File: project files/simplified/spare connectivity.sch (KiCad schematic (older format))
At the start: 4 parts, among them J6 Target STDC-14, U3 STM32F103CBUx

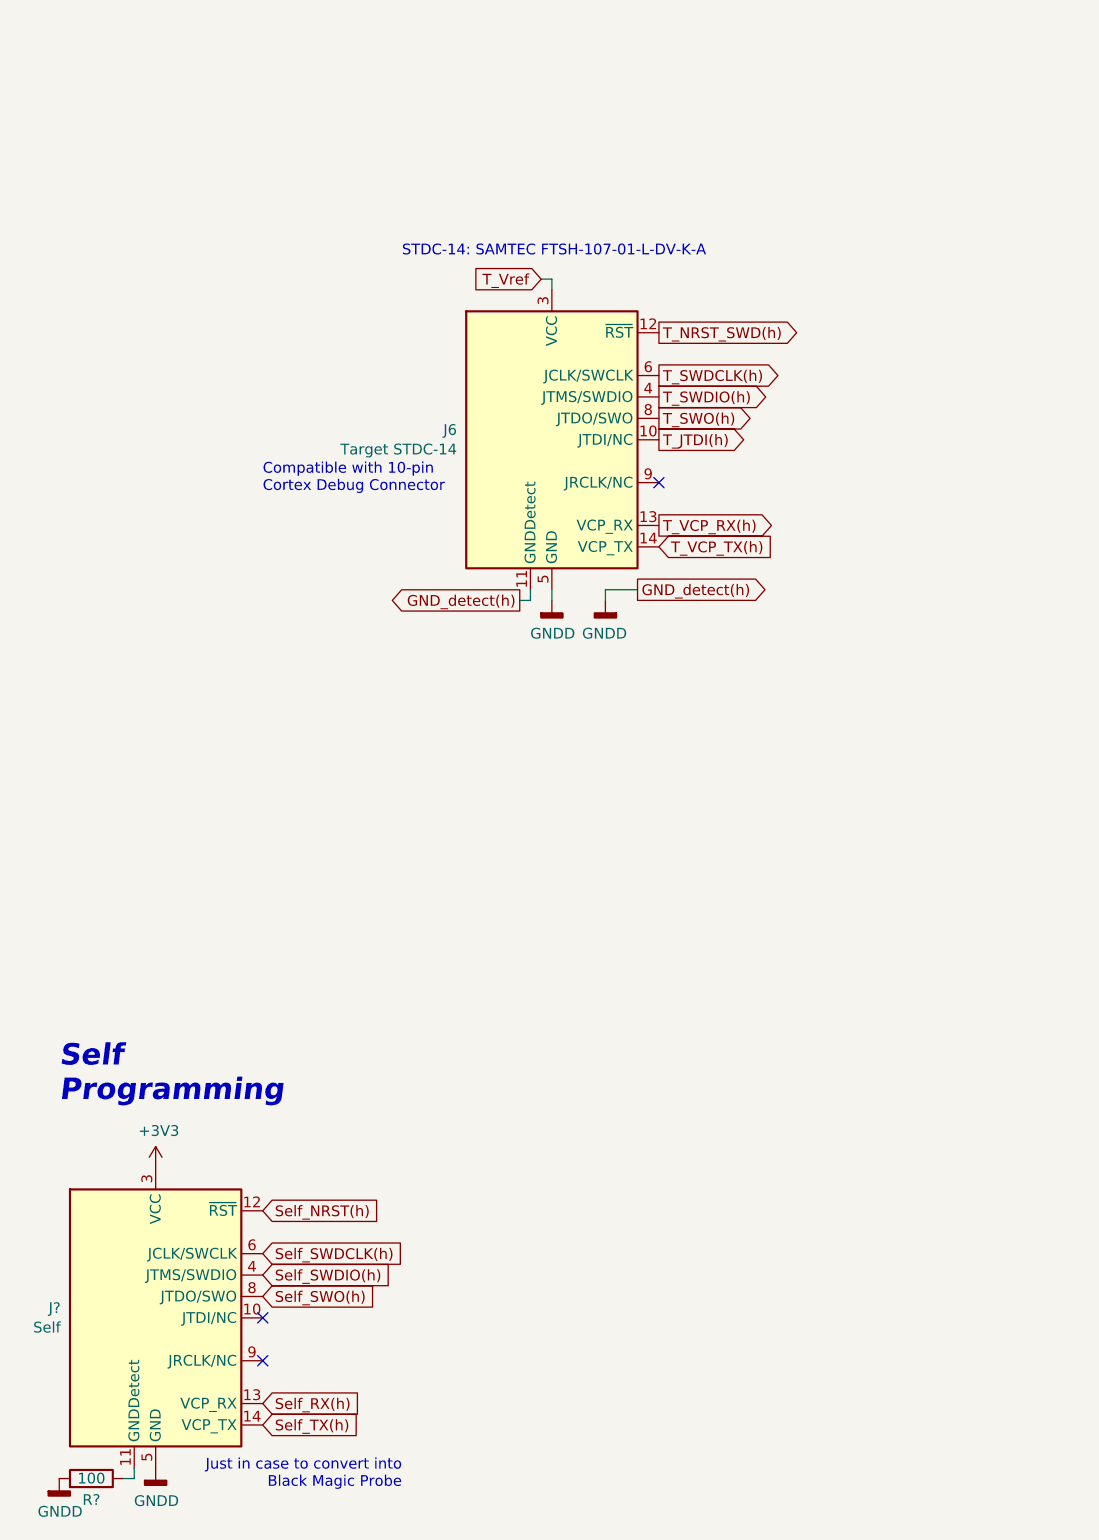
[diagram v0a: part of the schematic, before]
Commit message: re-arrangements
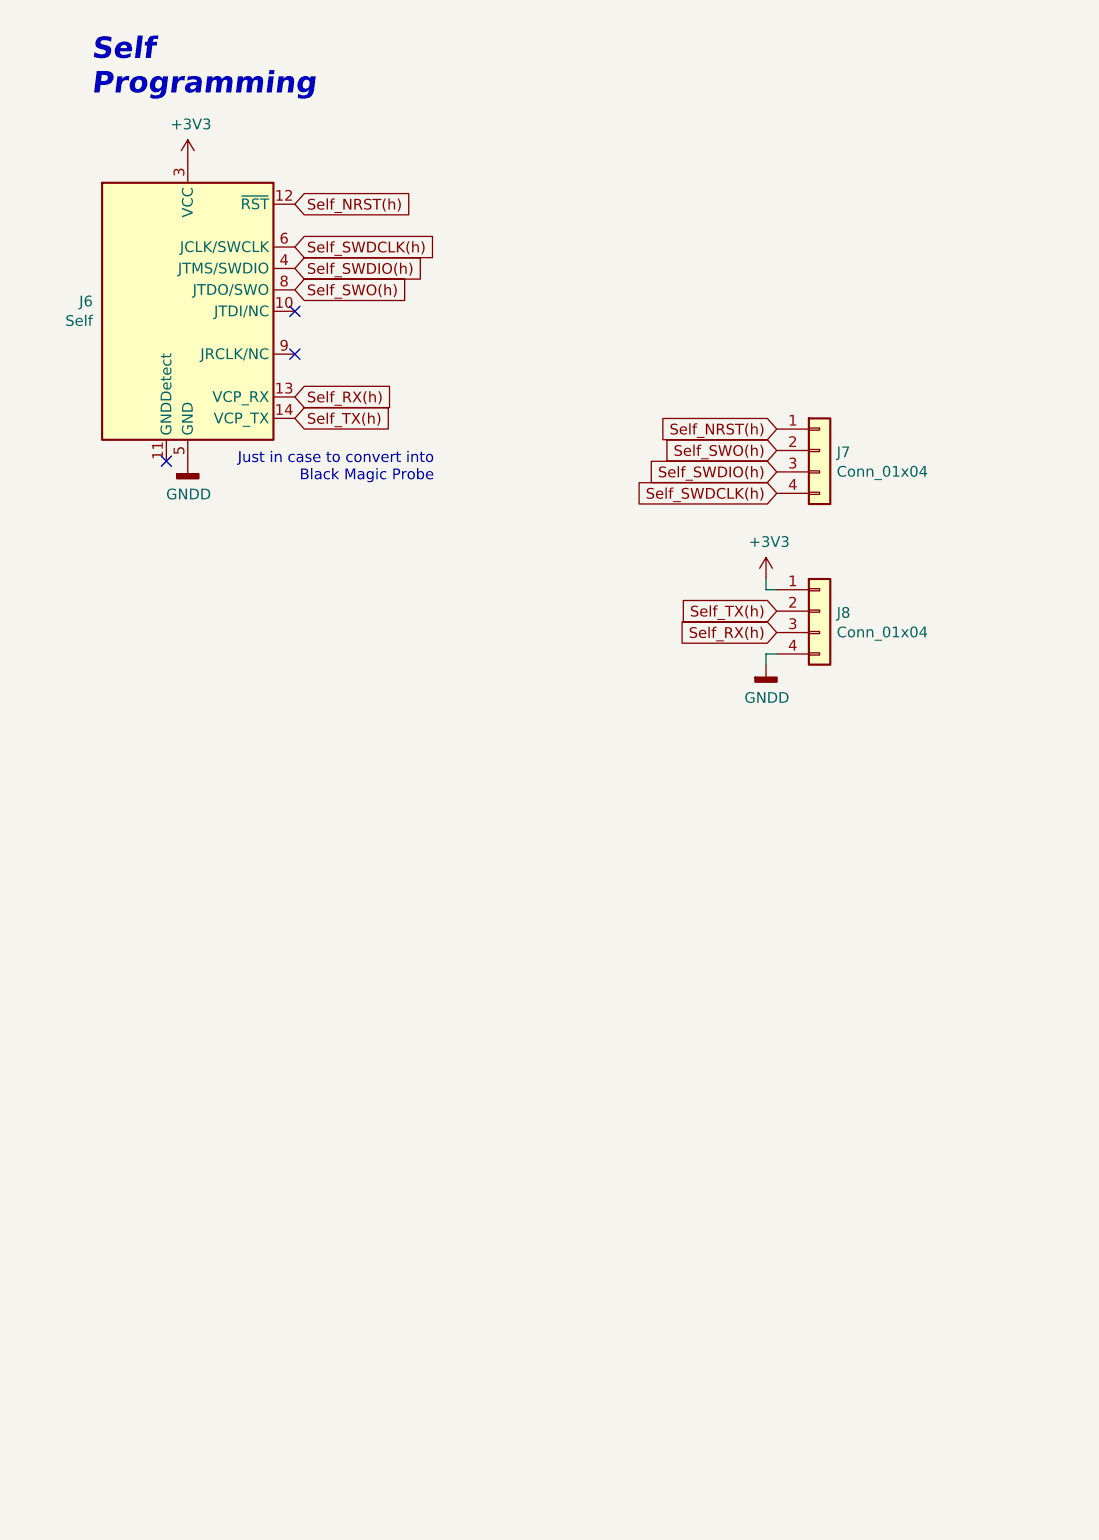
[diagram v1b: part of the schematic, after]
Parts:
- removed J6: Target STDC-14, Connector_PinHeader_1.27mm:PinHeader_2x07_P1.27mm_Vertical_SMD, symbol Connector:Conn_ST_STDC14
- removed R?: 100, Resistor_SMD:R_0603_1608Metric, symbol Device:R
- added J7, J8: Conn_01x04, Connector_PinHeader_2.54mm:PinHeader_1x04_P2.54mm_Vertical, symbol Connector_Generic:Conn_01x04
- gave numbers to parts that had none: 1
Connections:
- net +3V3: now also J8.1 (Pin_1)
- net GNDD: now also J8.4 (Pin_4)
- net Self_NRST(h): now also J7.1 (Pin_1)
- net Self_RX(h): now also J8.3 (Pin_3)
- net Self_SWDCLK(h): now also J7.4 (Pin_4)
- net Self_SWDIO(h): now also J7.3 (Pin_3)
- net Self_SWO(h): now also J7.2 (Pin_2)
- net Self_TX(h): now also J8.2 (Pin_2)
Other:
- note removed: "Compatible with 10-pin\nCortex Debug Connector"
- note removed: "STDC-14: SAMTEC FTSH-107-01-L-DV-K-A"
- moved on the sheet: J6
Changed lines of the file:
@@
 Comment4 ""
 $EndDescr
-Text GLabel 3450 2550 2    50   Output ~ 0
-T_SWO(h)
-Text GLabel 3450 2350 2    50   Output ~ 0
-T_SWDCLK(h)
-Text GLabel 3450 2150 2    50   Output ~ 0
-T_NRST_SWD(h)
-Text GLabel 3450 3150 2    50   Input ~ 0
-T_VCP_TX(h)
-Text GLabel 3450 3050 2    50   Output ~ 0
-T_VCP_RX(h)
-Text Notes 1600 2900 0    50   ~ 0
-Compatible with 10-pin\nCortex Debug Connector
-Text GLabel 3450 2450 2    50   Output ~ 0
-T_SWDIO(h)
-$Comp
-L power:GNDD #PWR?
-U 1 1 5EC35CB1
-P 2950 3400
-AR Path="/5EC35CB1" Ref="#PWR?"  Part="1"
-AR Path="/5EC31CA9/5EC35CB1" Ref="#PWR050"  Part="1"
-F 0 "#PWR050" H 2950 3150 50  0001 C CNN
-F 1 "GNDD" H 2954 3245 50  0000 C CNN
-F 2 "" H 2950 3400 50  0001 C CNN
-F 3 "" H 2950 3400 50  0001 C CNN
-	1    2950 3400
-	1    0    0    -1
-$EndComp
-Text Notes 2250 1800 0    50   ~ 0
-STDC-14: SAMTEC FTSH-107-01-L-DV-K-A
-$Comp
-L power:GNDD #PWR?
-U 1 1 5EC35CBA
-P 3200 3400
-AR Path="/5EC35CBA" Ref="#PWR?"  Part="1"
-AR Path="/5EC31CA9/5EC35CBA" Ref="#PWR051"  Part="1"
-F 0 "#PWR051" H 3200 3150 50  0001 C CNN
-F 1 "GNDD" H 3204 3245 50  0000 C CNN
-F 2 "" H 3200 3400 50  0001 C CNN
-F 3 "" H 3200 3400 50  0001 C CNN
-	1    3200 3400
-	-1   0    0    -1
-$EndComp
-Wire Wire Line
-	3350 3350 3200 3350
-Wire Wire Line
-	3200 3350 3200 3400
-Wire Wire Line
-	2800 3400 2850 3400
-Wire Wire Line
-	2850 3400 2850 3350
-Wire Wire Line
-	2950 3400 2950 3350
-NoConn ~ 3450 2850
-Text GLabel 3450 2650 2    50   Output ~ 0
-T_JTDI(h)
-$Comp
-L Connector:Conn_ST_STDC14 J?
-U 1 1 5EC35CC7
-P 2950 2650
-AR Path="/5EC35CC7" Ref="J?"  Part="1"
-AR Path="/5EC31CA9/5EC35CC7" Ref="J6"  Part="1"
-F 0 "J6" H 2507 2696 50  0000 R CNN
-F 1 "Target STDC-14" H 2507 2605 50  0000 R CNN
-F 2 "Connector_PinHeader_1.27mm:PinHeader_2x07_P1.27mm_Vertical_SMD" H 2950 2650 50  0001 C CNN
-F 3 "https://www.st.com/content/ccc/resource/technical/document/user_manual/group1/99/49/91/b6/b2/3a/46/e5/DM00526767/files/DM00526767.pdf/jcr:content/translations/en.DM00526767.pdf" V 2600 1400 50  0001 C CNN
-	1    2950 2650
-	1    0    0    -1
-$EndComp
-Wire Wire Line
-	2900 1900 2950 1900
-Wire Wire Line
-	2950 1900 2950 1950
-Text GLabel 2900 1900 0    50   Input ~ 0
-T_Vref
 Wire Wire Line
 	10050 4000 10050 3950
@@
 	9650 4000 9750 4000
 $Comp
-L power:GNDD #PWR053
+L power:GNDD #PWR055
 U 1 1 5EC6BDFB
 P 10050 4050
-F 0 "#PWR053" H 10050 3800 50  0001 C CNN
+F 0 "#PWR055" H 10050 3800 50  0001 C CNN
 F 1 "GNDD" H 10054 3895 50  0000 C CNN
 F 2 "" H 10050 4050 50  0001 C CNN
@@
 	9950 900  10050 900
 $Comp
-L power:+3.3V #PWR052
+L power:+3.3V #PWR050
 U 1 1 5EC6FD9F
 P 9850 900
-F 0 "#PWR052" H 9850 750 50  0001 C CNN
+F 0 "#PWR050" H 9850 750 50  0001 C CNN
 F 1 "+3.3V" H 9865 1073 50  0000 C CNN
 F 2 "" H 9850 900 50  0001 C CNN
@@
 	1    0    0    -1
 $EndComp
-Text GLabel 3350 3350 2    50   Output ~ 0
-GND_detect(h)
-Text GLabel 2800 3400 0    50   Output ~ 0
-GND_detect(h)
-Text Notes 2250 7550 2    50   ~ 0
+Text Notes 2400 2850 2    50   ~ 0
 Just in case to convert into\nBlack Magic Probe
-Text GLabel 1600 7250 2    50   Input ~ 0
+Text GLabel 1750 2550 2    50   Input ~ 0
 Self_TX(h)
-Text GLabel 1600 7150 2    50   Input ~ 0
+Text GLabel 1750 2450 2    50   Input ~ 0
 Self_RX(h)
 $Comp
-L power:GNDD #PWR?
+L power:GNDD #PWR052
 U 1 1 5F1BD152
-P 1100 7450
-F 0 "#PWR?" H 1100 7200 50  0001 C CNN
-F 1 "GNDD" H 1104 7295 50  0000 C CNN
-F 2 "" H 1100 7450 50  0001 C CNN
-F 3 "" H 1100 7450 50  0001 C CNN
-	1    1100 7450
-	1    0    0    -1
-$EndComp
-Text GLabel 1600 6250 2    50   Input ~ 0
+P 1250 2750
+F 0 "#PWR052" H 1250 2500 50  0001 C CNN
+F 1 "GNDD" H 1254 2595 50  0000 C CNN
+F 2 "" H 1250 2750 50  0001 C CNN
+F 3 "" H 1250 2750 50  0001 C CNN
+	1    1250 2750
+	1    0    0    -1
+$EndComp
+Text GLabel 1750 1550 2    50   Input ~ 0
 Self_NRST(h)
-NoConn ~ 1600 6950
-Text GLabel 1600 6650 2    50   Input ~ 0
+NoConn ~ 1750 2250
+Text GLabel 1750 1950 2    50   Input ~ 0
 Self_SWO(h)
-Text GLabel 1600 6450 2    50   Input ~ 0
+Text GLabel 1750 1750 2    50   Input ~ 0
 Self_SWDCLK(h)
-Text GLabel 1600 6550 2    50   Input ~ 0
+Text GLabel 1750 1850 2    50   Input ~ 0
 Self_SWDIO(h)
 $Comp
-L power:+3V3 #PWR?
+L power:+3V3 #PWR051
 U 1 1 5F1BD15D
-P 1100 6050
-F 0 "#PWR?" H 1100 5900 50  0001 C CNN
-F 1 "+3V3" H 1115 6223 50  0000 C CNN
-F 2 "" H 1100 6050 50  0001 C CNN
-F 3 "" H 1100 6050 50  0001 C CNN
-	1    1100 6050
-	1    0    0    -1
-$EndComp
-NoConn ~ 1600 6750
-$Comp
-L Connector:Conn_ST_STDC14 J?
+P 1250 1350
+F 0 "#PWR051" H 1250 1200 50  0001 C CNN
+F 1 "+3V3" H 1265 1523 50  0000 C CNN
+F 2 "" H 1250 1350 50  0001 C CNN
+F 3 "" H 1250 1350 50  0001 C CNN
+	1    1250 1350
+	1    0    0    -1
+$EndComp
+NoConn ~ 1750 2050
+$Comp
+L Connector:Conn_ST_STDC14 J6
 U 1 1 5F1BD164
-P 1100 6750
-F 0 "J?" H 657 6796 50  0000 R CNN
-F 1 "Self" H 657 6705 50  0000 R CNN
-F 2 "Connector_PinHeader_1.27mm:PinHeader_2x07_P1.27mm_Vertical_SMD" H 1100 6750 50  0001 C CNN
-F 3 "https://www.st.com/content/ccc/resource/technical/document/user_manual/group1/99/49/91/b6/b2/3a/46/e5/DM00526767/files/DM00526767.pdf/jcr:content/translations/en.DM00526767.pdf" V 750 5500 50  0001 C CNN
-	1    1100 6750
-	1    0    0    -1
-$EndComp
-Text Notes 650  5750 0    100  Italic 20
+P 1250 2050
+F 0 "J6" H 807 2096 50  0000 R CNN
+F 1 "Self" H 807 2005 50  0000 R CNN
+F 2 "Connector_PinHeader_1.27mm:PinHeader_2x07_P1.27mm_Vertical_SMD" H 1250 2050 50  0001 C CNN
+F 3 "https://www.st.com/content/ccc/resource/technical/document/user_manual/group1/99/49/91/b6/b2/3a/46/e5/DM00526767/files/DM00526767.pdf/jcr:content/translations/en.DM00526767.pdf" V 900 800 50  0001 C CNN
+	1    1250 2050
+	1    0    0    -1
+$EndComp
+Text Notes 800  1050 0    100  Italic 20
 Self\nProgramming
-$Comp
-L Device:R R?
-U 1 1 5F1BD16B
-P 800 7500
-F 0 "R?" V 700 7500 50  0000 C CNN
-F 1 "100" V 800 7500 50  0000 C CNN
-F 2 "Resistor_SMD:R_0603_1608Metric" V 730 7500 50  0001 C CNN
-F 3 "~" H 800 7500 50  0001 C CNN
-	1    800  7500
-	0    1    -1   0
-$EndComp
-$Comp
-L power:GNDD #PWR?
-U 1 1 5F1BD171
-P 650 7500
-F 0 "#PWR?" H 650 7250 50  0001 C CNN
-F 1 "GNDD" H 654 7345 50  0000 C CNN
-F 2 "" H 650 7500 50  0001 C CNN
-F 3 "" H 650 7500 50  0001 C CNN
-	1    650  7500
-	1    0    0    -1
-$EndComp
-Wire Wire Line
-	950  7500 1000 7500
-Wire Wire Line
-	1000 7500 1000 7450
+NoConn ~ 1150 2750
+$Comp
+L Connector_Generic:Conn_01x04 J7
+U 1 1 5FCDFBAC
+P 4200 2700
+F 0 "J7" H 4280 2692 50  0000 L CNN
+F 1 "Conn_01x04" H 4280 2601 50  0000 L CNN
+F 2 "Connector_PinHeader_2.54mm:PinHeader_1x04_P2.54mm_Vertical" H 4200 2700 50  0001 C CNN
+F 3 "~" H 4200 2700 50  0001 C CNN
+	1    4200 2700
+	1    0    0    -1
+$EndComp
+$Comp
+L Connector_Generic:Conn_01x04 J8
+U 1 1 5FCE032D
+P 4200 3450
+F 0 "J8" H 4280 3442 50  0000 L CNN
+F 1 "Conn_01x04" H 4280 3351 50  0000 L CNN
+F 2 "Connector_PinHeader_2.54mm:PinHeader_1x04_P2.54mm_Vertical" H 4200 3450 50  0001 C CNN
+F 3 "~" H 4200 3450 50  0001 C CNN
+	1    4200 3450
+	1    0    0    -1
+$EndComp
+Text GLabel 4000 3450 0    50   Input ~ 0
+Self_TX(h)
+Text GLabel 4000 3550 0    50   Input ~ 0
+Self_RX(h)
+$Comp
+L power:GNDD #PWR054
+U 1 1 5FCE1122
+P 3950 3700
+F 0 "#PWR054" H 3950 3450 50  0001 C CNN
+F 1 "GNDD" H 3954 3545 50  0000 C CNN
+F 2 "" H 3950 3700 50  0001 C CNN
+F 3 "" H 3950 3700 50  0001 C CNN
+	1    3950 3700
+	1    0    0    -1
+$EndComp
+$Comp
+L power:+3V3 #PWR053
+U 1 1 5FCE1839
+P 3950 3300
+F 0 "#PWR053" H 3950 3150 50  0001 C CNN
+F 1 "+3V3" H 3965 3473 50  0000 C CNN
+F 2 "" H 3950 3300 50  0001 C CNN
+F 3 "" H 3950 3300 50  0001 C CNN
+	1    3950 3300
+	1    0    0    -1
+$EndComp
+Wire Wire Line
+	4000 3350 3950 3350
+Wire Wire Line
+	3950 3350 3950 3300
+Wire Wire Line
+	4000 3650 3950 3650
+Wire Wire Line
+	3950 3650 3950 3700
+Text GLabel 4000 2700 0    50   Input ~ 0
+Self_SWO(h)
+Text GLabel 4000 2900 0    50   Input ~ 0
+Self_SWDCLK(h)
+Text GLabel 4000 2800 0    50   Input ~ 0
+Self_SWDIO(h)
+Text GLabel 4000 2600 0    50   Input ~ 0
+Self_NRST(h)
 $EndSCHEMATC

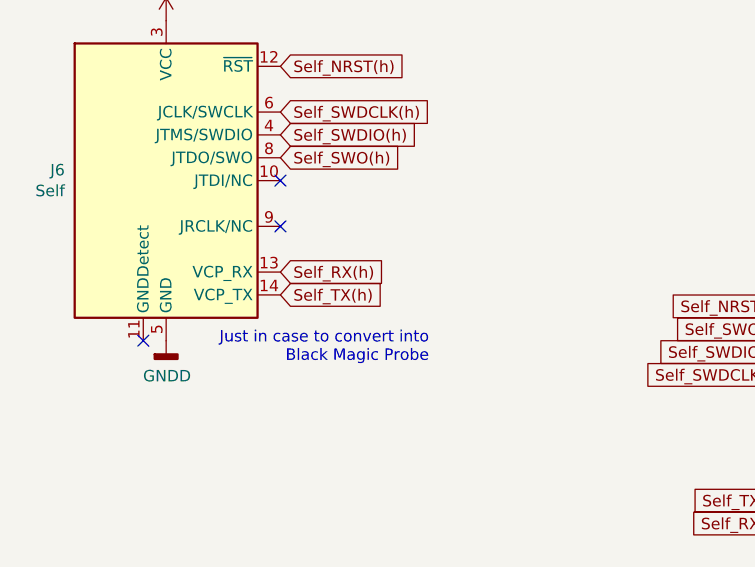
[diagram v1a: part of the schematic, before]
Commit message: Self RX/TX fix
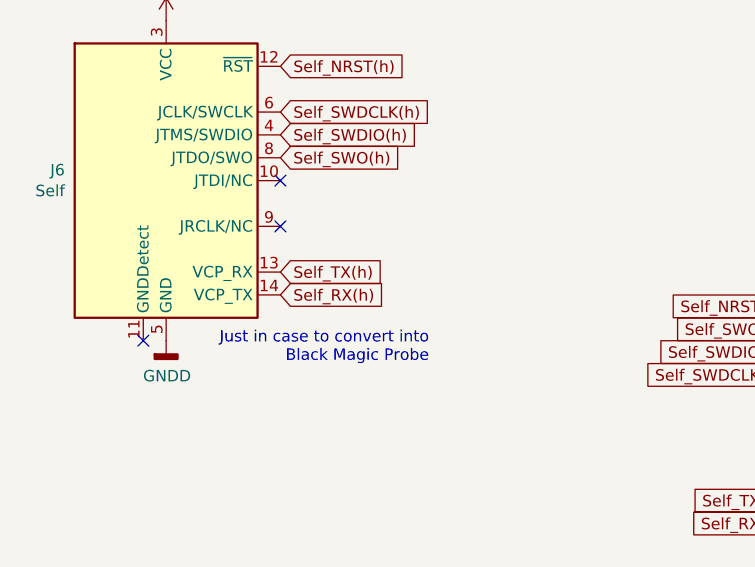
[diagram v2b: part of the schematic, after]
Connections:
- net Self_RX(h): now also J6.14 (VCP_TX); no longer J6.13 (VCP_RX)
- net Self_TX(h): now also J6.13 (VCP_RX); no longer J6.14 (VCP_TX)
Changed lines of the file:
@@
 Text Notes 2400 2850 2    50   ~ 0
 Just in case to convert into\nBlack Magic Probe
+Text GLabel 1750 2450 2    50   Input ~ 0
+Self_TX(h)
 Text GLabel 1750 2550 2    50   Input ~ 0
-Self_TX(h)
-Text GLabel 1750 2450 2    50   Input ~ 0
 Self_RX(h)
 $Comp
